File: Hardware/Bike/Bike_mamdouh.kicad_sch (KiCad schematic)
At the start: 19 parts, among them U1 ESP32-WROOM-32

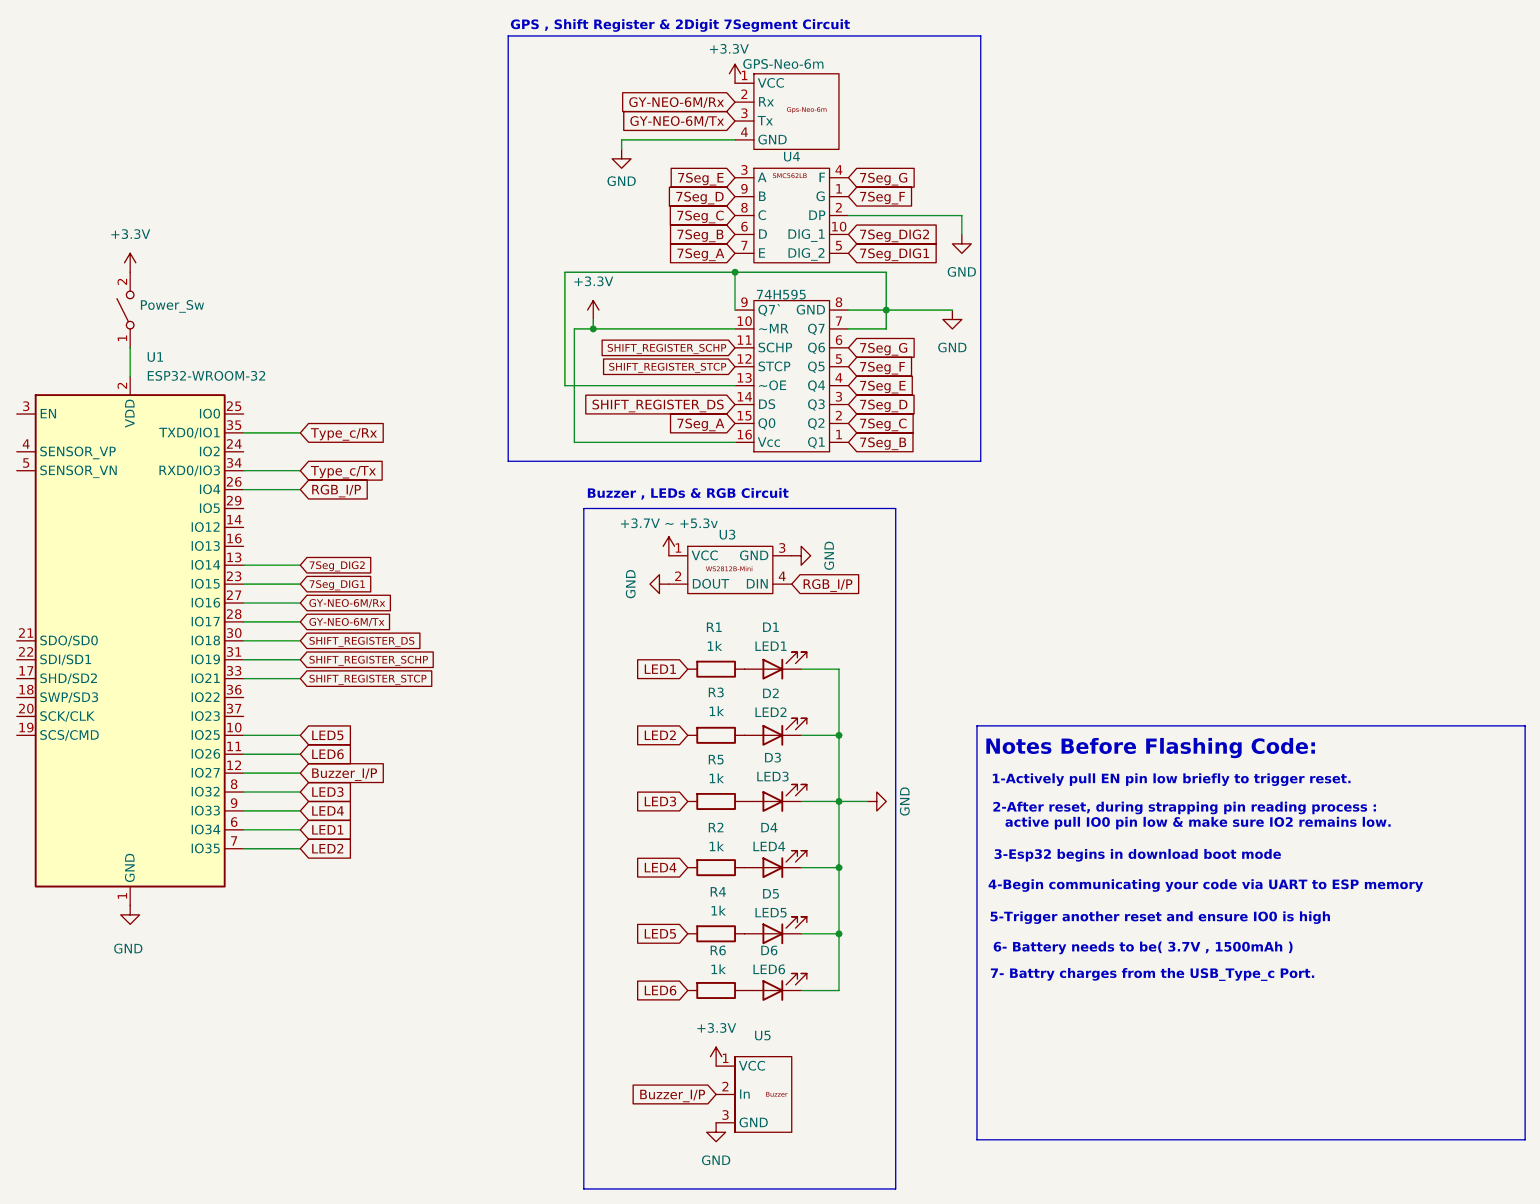
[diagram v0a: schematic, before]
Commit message: fixing testing note
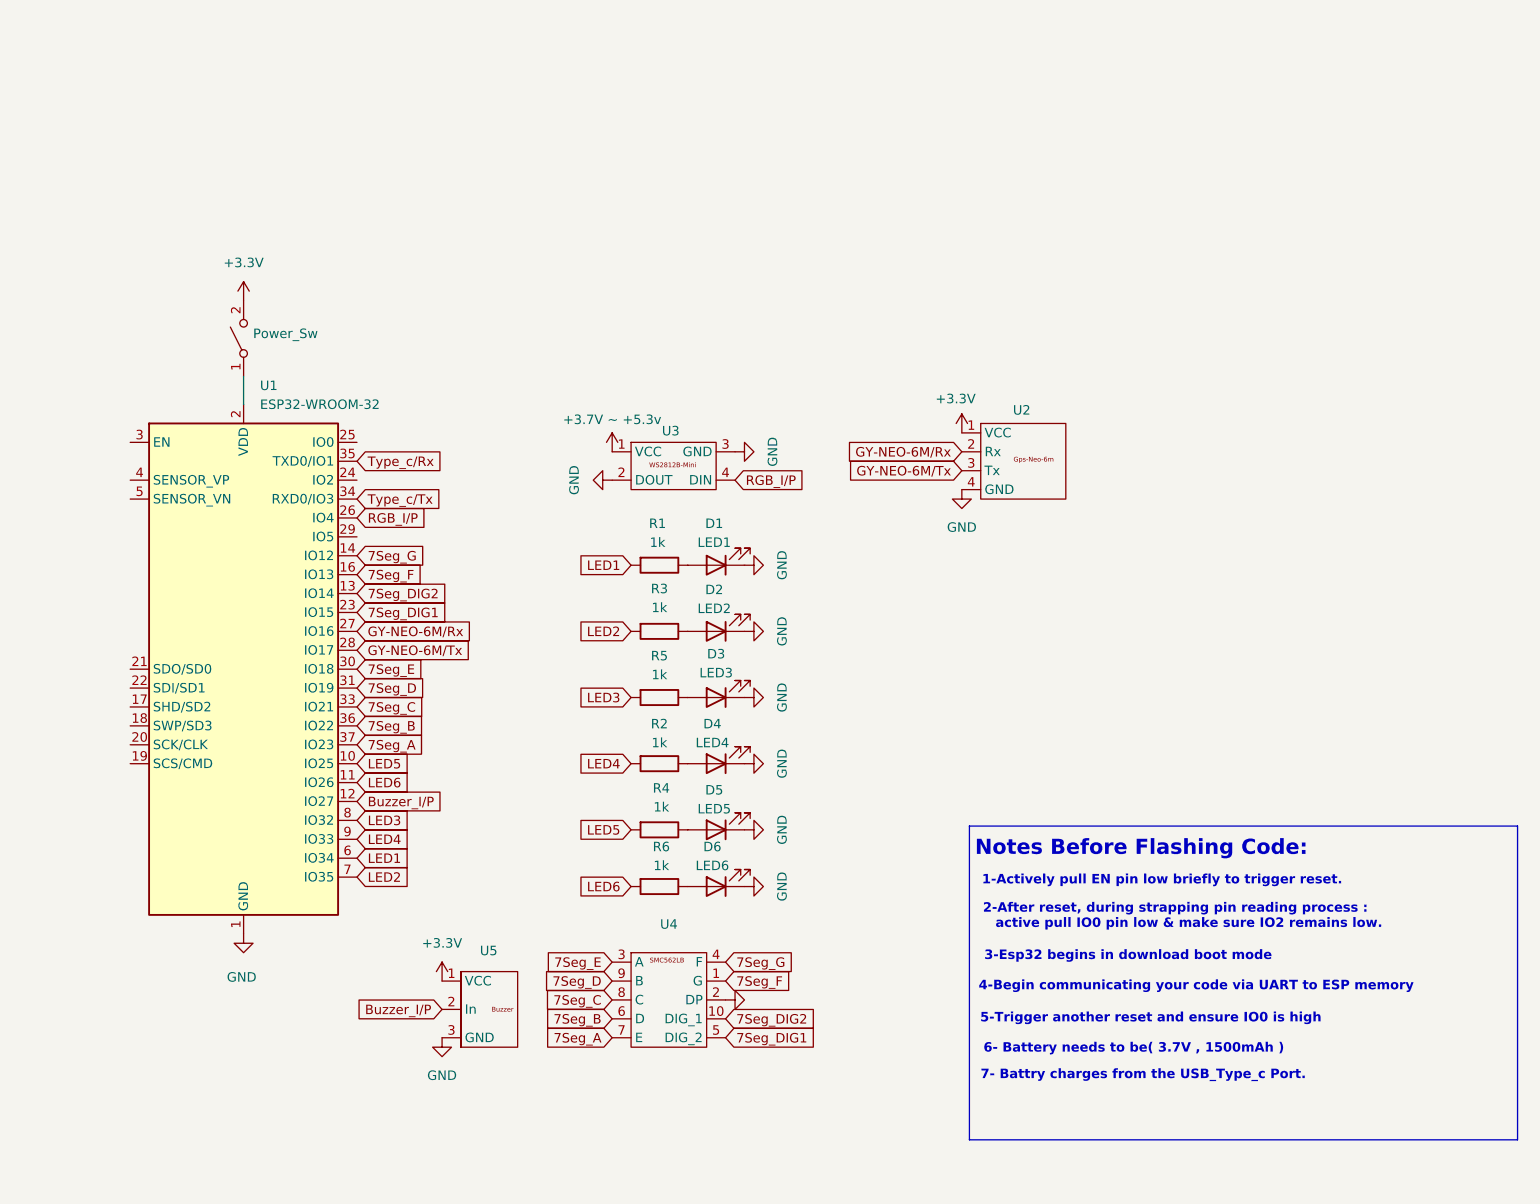
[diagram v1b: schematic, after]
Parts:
- removed 74H595: ~, symbol Shift-register-74H595:74H595
- renumbered GPS-Neo-6m to U2
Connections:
- net SHIFT_REGISTER_DS is gone; now on net 7Seg_E: U1.30 (IO18)
- net SHIFT_REGISTER_SCHP is gone; now on net 7Seg_D: U1.31 (IO19)
- net SHIFT_REGISTER_STCP is gone; now on net 7Seg_C: U1.33 (IO21)
- net 7Seg_A: now also U1.37 (IO23)
- net 7Seg_B: now also U1.36 (IO22)
- net 7Seg_F: now also U1.16 (IO13)
- net 7Seg_G: now also U1.14 (IO12)
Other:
- note removed: "Buzzer , LEDs & RGB Circuit"
- note removed: "GPS , Shift Register & 2Digit 7Segment Circuit"
- moved on the sheet: D1, D2, D3, D4, D5, D6, Power_Sw, R1, R2, R3, R4, R5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
